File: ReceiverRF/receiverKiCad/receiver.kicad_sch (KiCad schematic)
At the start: 23 parts, among them U1 STM32F103RET6, Y1 Crystal_GND24

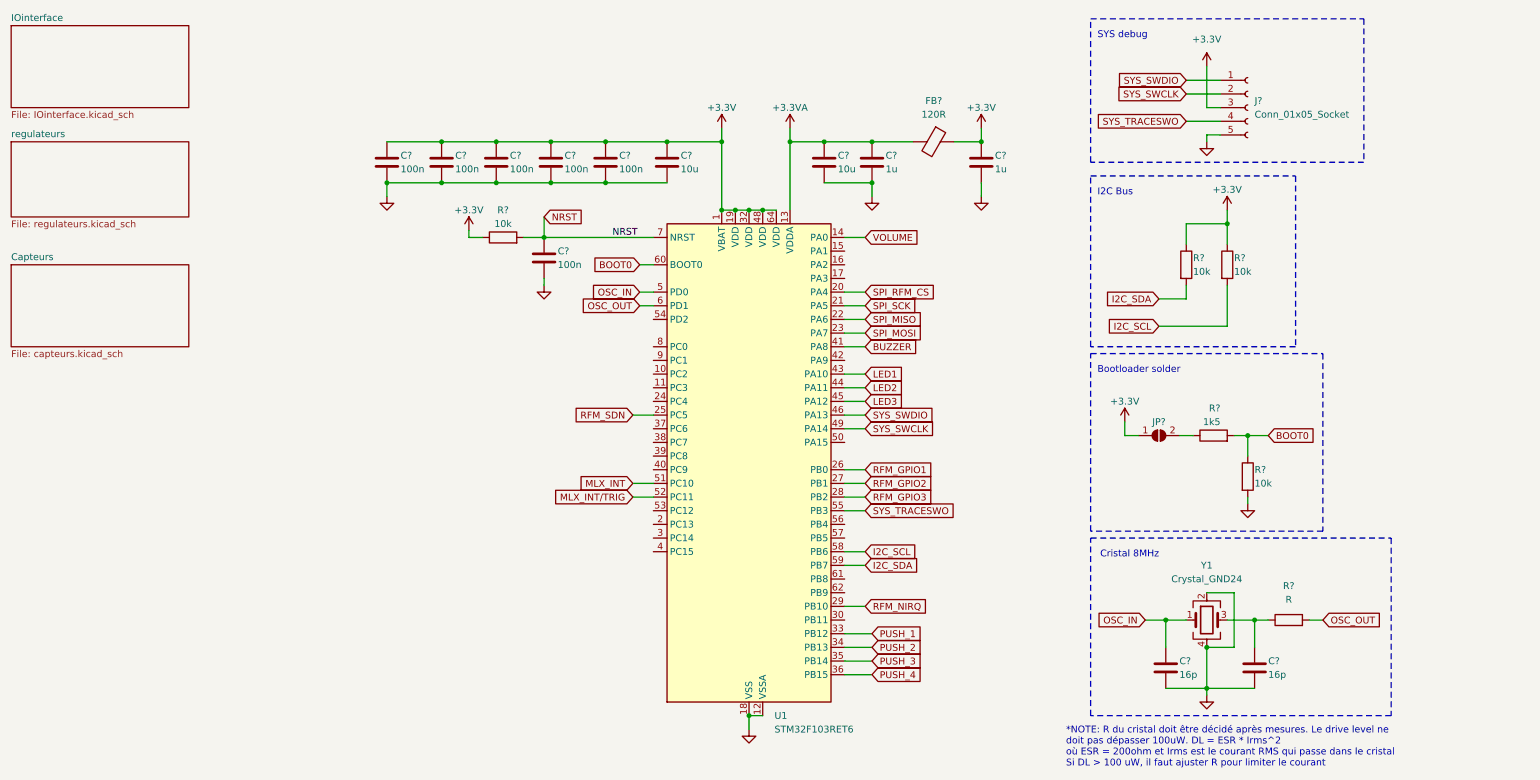
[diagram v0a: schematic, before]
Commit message: Identifiants des symboles
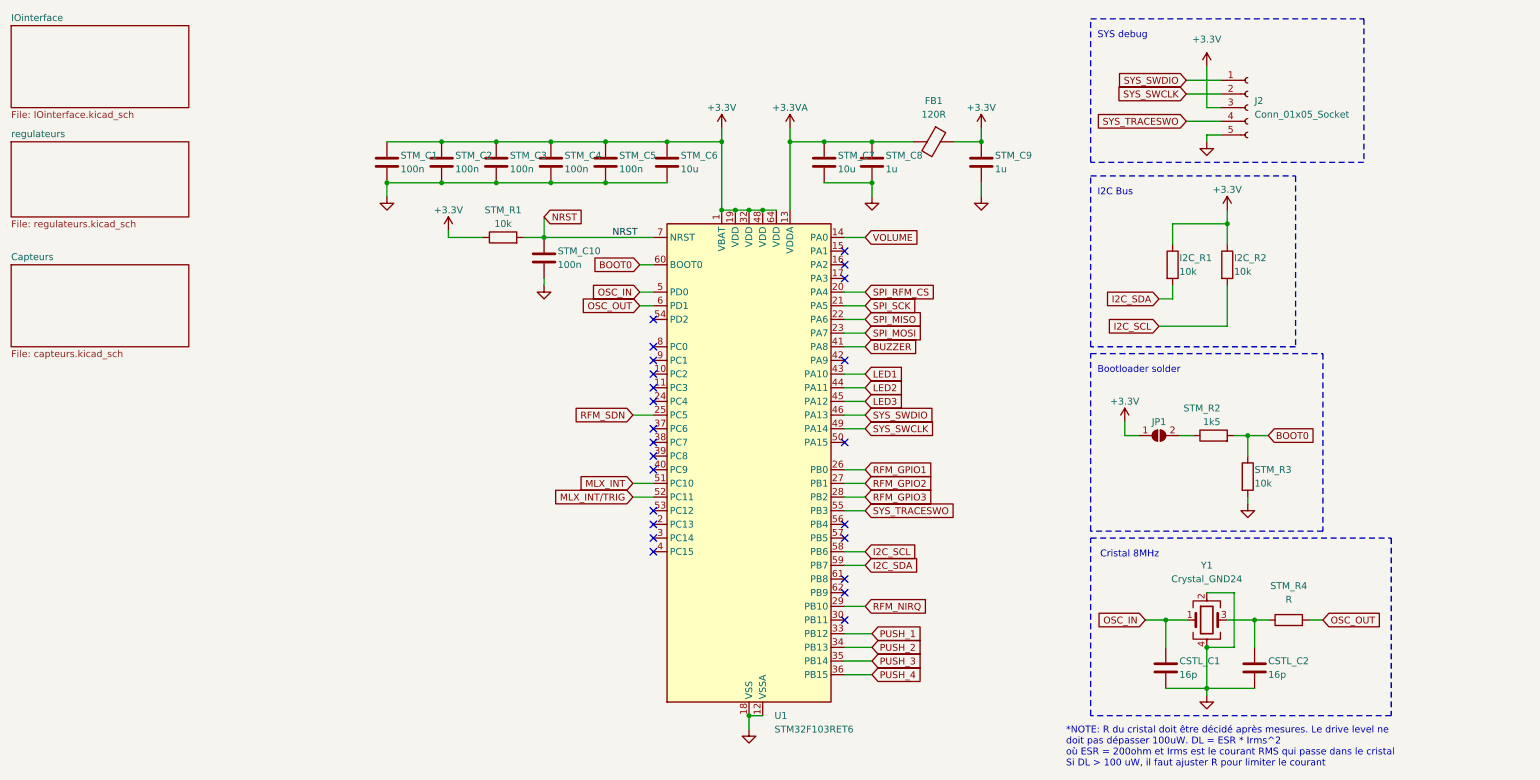
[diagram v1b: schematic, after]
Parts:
- gave numbers to parts that had none: 21
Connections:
- no-connect marks 0 -> 24
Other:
- moved on the sheet: I2C_R1
